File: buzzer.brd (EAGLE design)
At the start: 13 x 36.3 mm, 3 parts

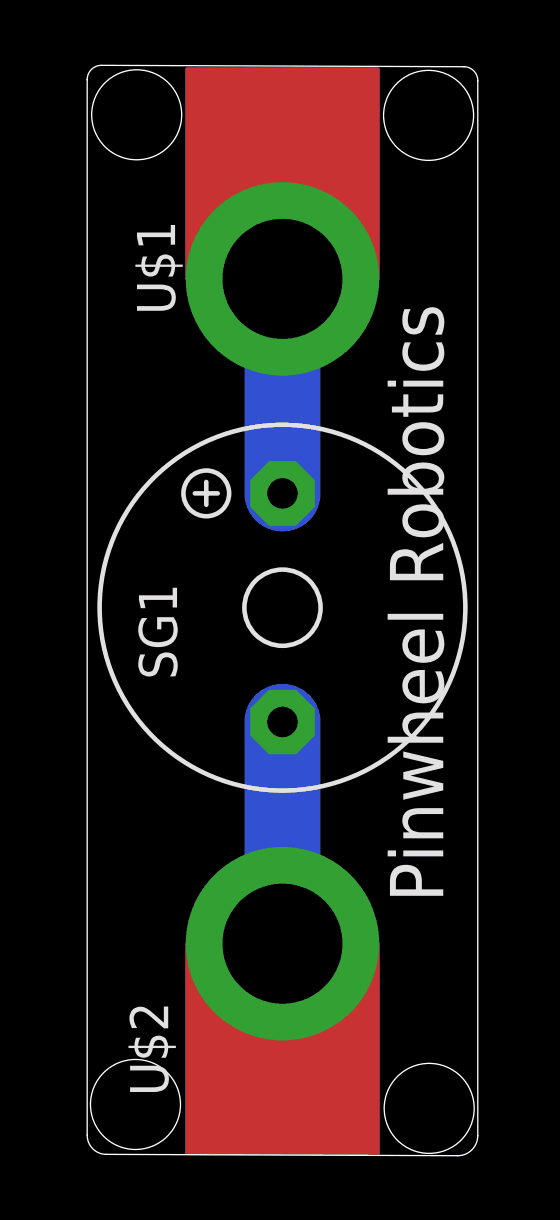
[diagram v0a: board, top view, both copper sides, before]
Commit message: New Updates
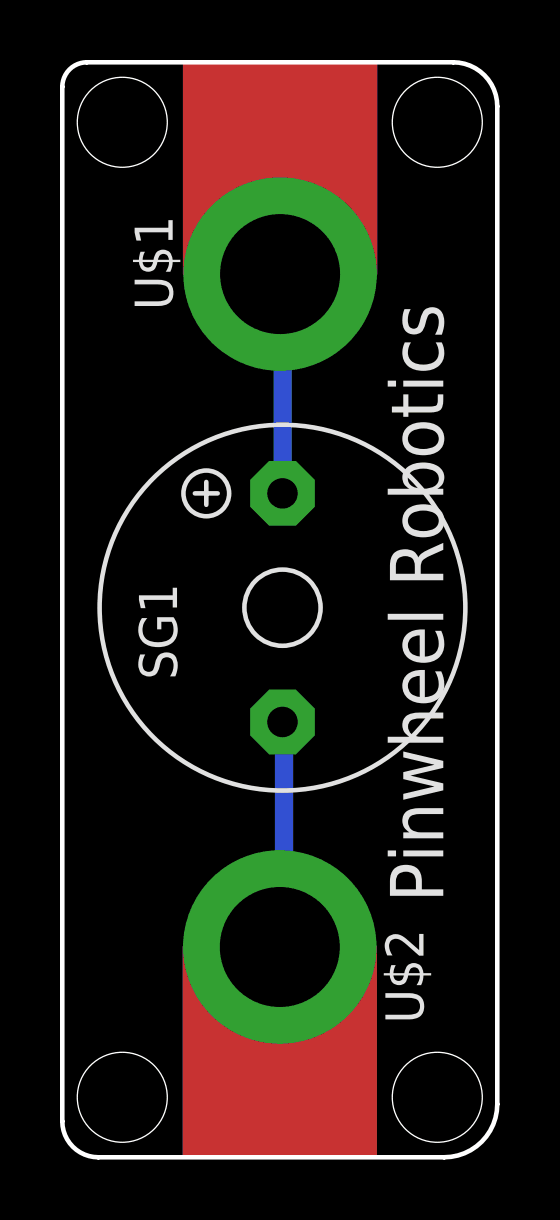
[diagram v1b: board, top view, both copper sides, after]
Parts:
- moved U$1 0.18 mm to (15.3, 31.4)
- moved U$2 0.14 mm to (15.2, 9.01)
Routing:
- net N$2: track 11.0 -> 7.58 mm
- net N$1: track 10.4 -> 7.86 mm
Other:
- board size 13 x 36.3 mm -> 14.5 x 36.5 mm
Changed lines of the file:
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@@
 <setting verticaltext="up"/>
 </settings>
-<grid distance="0.1" unitdist="mm" unit="mm" style="lines" multiple="1" display="yes" altdistance="0.01" altunitdist="mm" altunit="mm"/>
+<grid distance="0.5" unitdist="mm" unit="mm" style="lines" multiple="1" display="yes" altdistance="0.01" altunitdist="mm" altunit="mm"/>
 <layers>
 <layer number="1" name="Top" color="4" fill="1" visible="yes" active="yes"/>
@@
 <board>
 <plain>
-<wire x1="8.83" y1="37.923321875" x2="8.83" y2="2.732328125" width="0" layer="20"/>
-<wire x1="8.83" y1="2.732328125" x2="9.462325" y2="2.097571875" width="0" layer="20" curve="89.779982"/>
-<wire x1="9.462325" y1="2.097571875" x2="21.1785125" y2="2.052578125" width="0" layer="20"/>
-<wire x1="21.1785125" y1="2.052578125" x2="21.85" y2="2.72149375" width="0" layer="20" curve="90.221368"/>
-<wire x1="21.85" y1="2.72149375" x2="21.85" y2="37.88914375" width="0" layer="20"/>
-<wire x1="21.85" y1="37.88914375" x2="21.38915" y2="38.35176875" width="0" layer="20" curve="89.779782"/>
-<wire x1="21.38915" y1="38.35176875" x2="9.306675" y2="38.39816875" width="0" layer="20"/>
-<wire x1="9.306675" y1="38.39816875" x2="8.83" y2="37.923321875" width="0" layer="20" curve="90.175163"/>
-<hole x="10.44" y="3.76" drill="3"/>
-<hole x="20.23" y="3.63" drill="3"/>
-<hole x="20.21" y="36.73" drill="3"/>
-<hole x="10.48" y="36.75" drill="3"/>
+<hole x="10" y="4" drill="3"/>
+<hole x="20.5" y="4" drill="3"/>
+<hole x="20.5" y="36.5" drill="3"/>
+<hole x="10" y="36.5" drill="3"/>
 <text x="20.7" y="10.5" size="1.778" layer="21" rot="R90">Pinwheel Robotics </text>
 <text x="11.3" y="28.9" size="1.778" layer="22" rot="MR270">care@Pinwheel.in</text>
+<wire x1="9.200715625" y1="2" x2="20.729509375" y2="2" width="0.1524" layer="20"/>
+<wire x1="20.729509375" y1="2" x2="22.5" y2="3.770490625" width="0.1524" layer="20" curve="90"/>
+<wire x1="22.5" y1="3.770490625" x2="22.5" y2="37.0320625" width="0.1524" layer="20"/>
+<wire x1="22.5" y1="37.0320625" x2="21.0320625" y2="38.5" width="0.1524" layer="20" curve="90"/>
+<wire x1="21.0320625" y1="38.5" x2="8.81941875" y2="38.5" width="0.1524" layer="20"/>
+<wire x1="8.81941875" y1="38.5" x2="8" y2="37.68058125" width="0.1524" layer="20" curve="90"/>
+<wire x1="8" y1="37.68058125" x2="8" y2="3.200715625" width="0.1524" layer="20"/>
+<wire x1="8" y1="3.200715625" x2="9.200715625" y2="2" width="0.1524" layer="20" curve="90"/>
 </plain>
 <attributes>
@@
 <autorouter>
 <pass name="Default">
-<param name="RoutingGrid" value="50mil"/>
+<param name="RoutingGrid" value="0.25mm"/>
 <param name="AutoGrid" value="1"/>
 <param name="Efforts" value="0"/>
@@
 <param name="PrefDir.14" value="0"/>
 <param name="PrefDir.15" value="0"/>
-<param name="PrefDir.16" value="a"/>
+<param name="PrefDir.16" value="-"/>
 <param name="cfVia" value="8"/>
 <param name="cfNonPref" value="5"/>
@@
 <attribute name="VALUE" x="18.34" y="18.22" size="1.27" layer="27" ratio="10" rot="R90"/>
 </element>
-<element name="U$1" library="microbit" package="MICROBIT_PAD" value="MICROBIT_PAD" x="15.34" y="31.28" smashed="yes" rot="R180">
-<attribute name="NAME" x="11.76" y="30.08" size="1.27" layer="21" rot="R90"/>
+<element name="U$1" library="microbit" package="MICROBIT_PAD" value="MICROBIT_PAD" x="15.26" y="31.44" smashed="yes" rot="R180">
+<attribute name="NAME" x="11.68" y="30.24" size="1.27" layer="21" rot="R90"/>
 </element>
-<element name="U$2" library="microbit" package="MICROBIT_PAD" value="MICROBIT_PAD" x="15.34" y="9.12" smashed="yes">
-<attribute name="NAME" x="11.53" y="4.04" size="1.27" layer="21" rot="R90"/>
+<element name="U$2" library="microbit" package="MICROBIT_PAD" value="MICROBIT_PAD" x="15.25" y="9.01" smashed="yes">
+<attribute name="NAME" x="20.04" y="6.46" size="1.27" layer="21" rot="R90"/>
 </element>
 </elements>
@@
 <contactref element="SG1" pad="+"/>
 <contactref element="U$1" pad="PAD"/>
-<wire x1="15.5448" y1="34.4424" x2="15.34" y2="34.2376" width="0.1524" layer="16"/>
-<wire x1="15.34" y1="31.28" x2="15.34" y2="34.2376" width="0.1524" layer="16"/>
-<wire x1="15.34" y1="24.13" x2="15.34" y2="31.28" width="2.54" layer="16"/>
+<wire x1="15.34" y1="24.605675" x2="15.34" y2="24.13" width="0.6096" layer="16"/>
+<wire x1="15.34" y1="24.605675" x2="15.33" y2="24.61" width="0.6096" layer="16"/>
+<wire x1="15.3448" y1="31.41079375" x2="15.3448" y2="24.6964" width="0.6096" layer="16"/>
+<wire x1="15.3448" y1="24.6964" x2="15.34" y2="24.686875" width="0.1524" layer="16"/>
+<wire x1="15.34" y1="24.686875" x2="15.34" y2="24.13" width="0.1524" layer="16"/>
+<wire x1="15.3448" y1="31.41079375" x2="15.26" y2="31.44" width="0.6096" layer="16"/>
 </signal>
 <signal name="N$2">
 <contactref element="SG1" pad="-"/>
 <contactref element="U$2" pad="PAD"/>
-<wire x1="14.917034375" y1="6.382634375" x2="14.6304" y2="6.096" width="0.1524" layer="16"/>
-<wire x1="14.917034375" y1="6.382634375" x2="15.34" y2="9.12" width="0.1524" layer="16"/>
-<wire x1="15.34" y1="16.51" x2="15.34" y2="9.36" width="2.54" layer="16"/>
-<wire x1="15.34" y1="9.36" x2="15.8" y2="8.9" width="2.54" layer="16"/>
-<wire x1="15.34" y1="9.12" x2="15.8" y2="8.9" width="0" layer="19" extent="16-16"/>
+<wire x1="15.3924" y1="9.144" x2="15.3924" y2="16.4592" width="0.6096" layer="16"/>
+<wire x1="15.3924" y1="16.4592" x2="15.34" y2="16.51" width="0.1524" layer="16"/>
+<wire x1="15.3924" y1="9.144" x2="15.25" y2="9.01" width="0.1524" layer="16"/>
 </signal>
 </signals>
